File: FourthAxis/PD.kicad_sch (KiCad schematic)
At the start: 2 parts, among them U3 XL1509-5.0, U4 XL1509-3.3

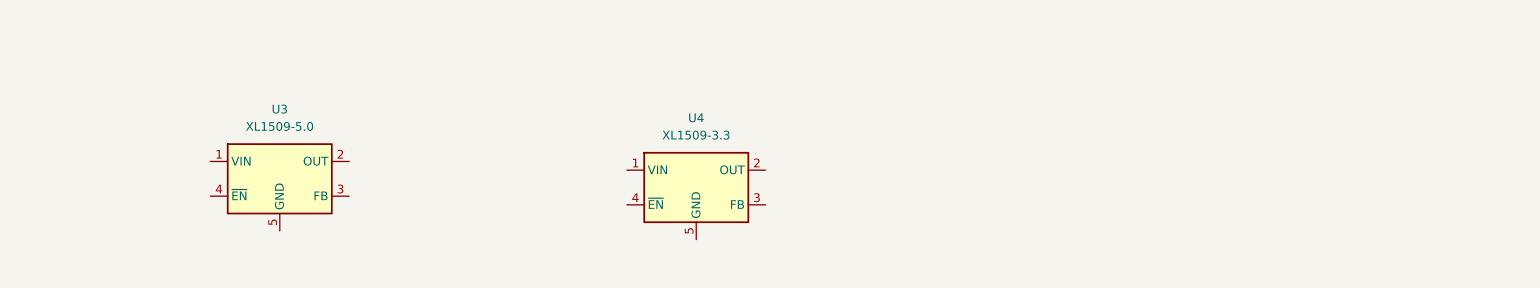
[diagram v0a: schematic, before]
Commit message: Shaun work
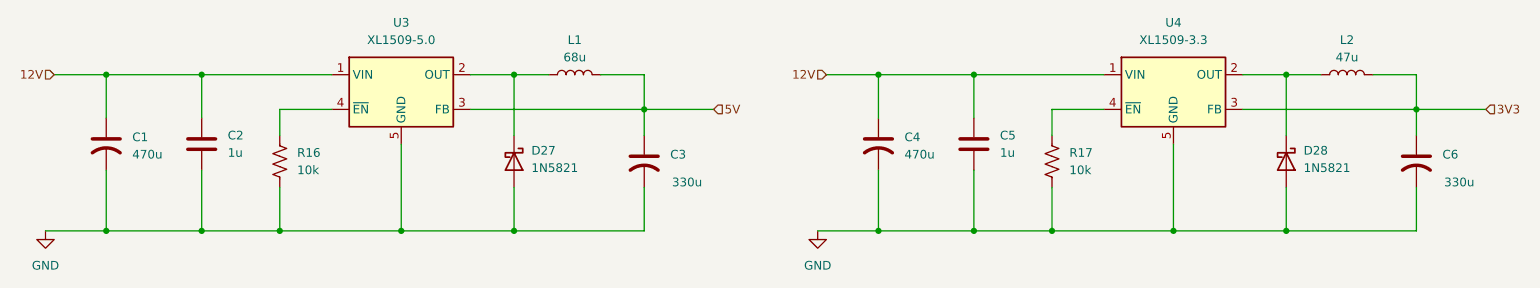
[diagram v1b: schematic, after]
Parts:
- added C1, C4: 470u, symbol Device:C_US
- added C2, C5: 1u, symbol Device:C
- added C3, C6: 330u, symbol Device:C_US
- added D27, D28: 1N5821, Diode_THT:D_DO-201AD_P15.24mm_Horizontal, symbol Diode:1N5821
- added L1: 68u, symbol Device:L
- added L2: 47u, symbol Device:L
- added R16, R17: 10k, symbol Device:R_US
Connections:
- net 12V: now reaches U3.1 (VIN)
- net 12V: now also U4.1 (VIN), C1.1, C2.1, C4.1, C5.1
- net at U3.2 (OUT): now also D27.1 (K), L1.1
- net 5V: now reaches U3.3 (FB)
- net 5V: now also C3.1, L1.2
- net at U3.4 (~{EN}): now also R16.1
- net GND: now reaches U3.5 (GND), U3.6 (GND), U3.7 (GND), U3.8 (GND)
- net GND: now also U4.5 (GND), U4.6 (GND), U4.7 (GND), U4.8 (GND), C1.2, C2.2, C3.2, C4.2, C5.2, C6.2, D27.2 (A), D28.2 (A), R16.2, R17.2
- net at U4.2 (OUT): now also D28.1 (K), L2.1
- net 3V3: now reaches U4.3 (FB)
- net 3V3: now also C6.1, L2.2
- net at U4.4 (~{EN}): now also R17.1
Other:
- moved on the sheet: U3, U4
